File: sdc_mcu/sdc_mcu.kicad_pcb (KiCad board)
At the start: 2 copper layers, 70 x 45 mm, 93 parts, among them J1 Conn_02x10_Odd_Even, K1 G2RL-2A, K2 G2RL-2A, K3 G2RL-2A, K4 G2RL-2A, Q1 2N7002, Q2 2N7002, Q3 2N7002, Q4 2N7002, Q5 2N7002, Q6 2N7002, U1 VOM618AT, U10 AP2204K-ADJ, U2 VOM618AT, U3 AS331KTR-G1, U4 AS331KTR-G1, U5 AS331KTR-G1, U6 VOM618AT, U7 VOM618AT, U9 AP2204K-ADJ

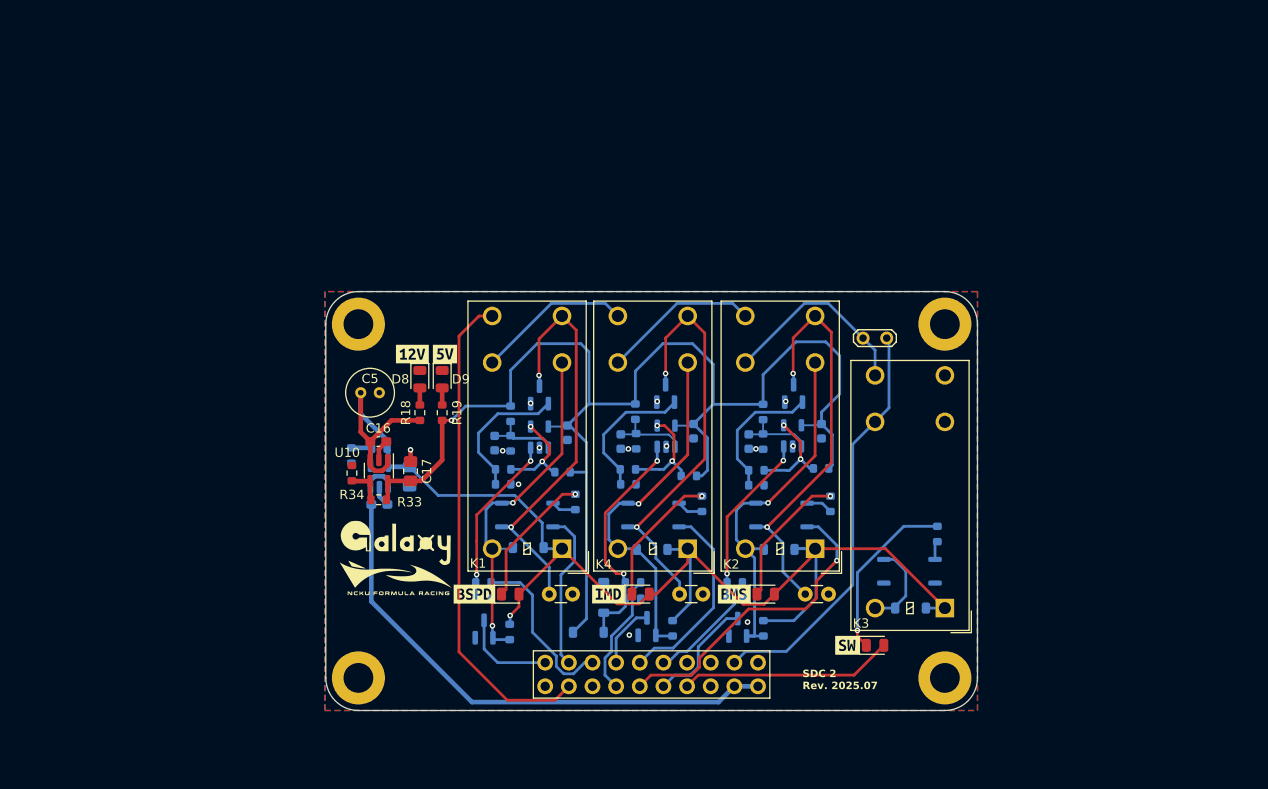
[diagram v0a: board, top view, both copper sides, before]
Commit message: v2025.10
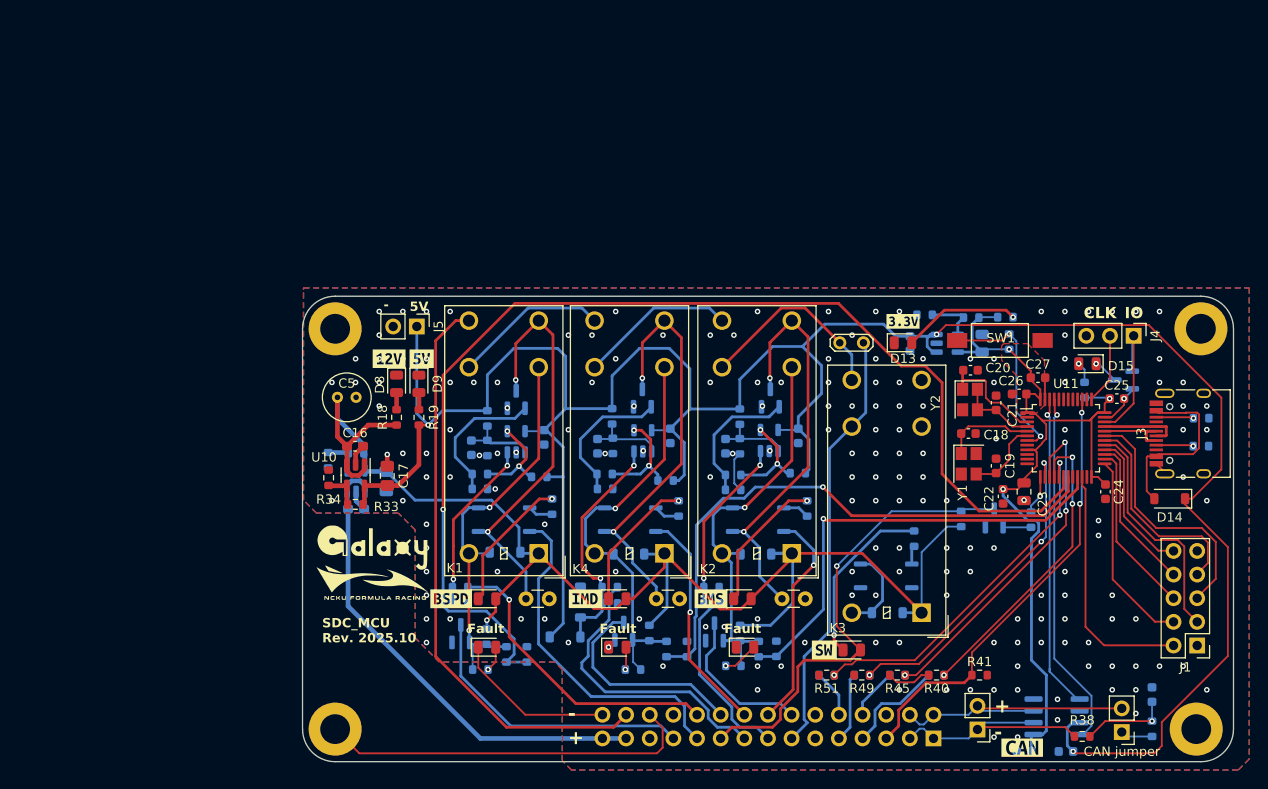
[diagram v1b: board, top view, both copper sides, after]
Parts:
- added C18: 20p, Capacitor_SMD:C_0603_1608Metric, F.Cu at (122.0, 63.2)
- added C19: 20p, Capacitor_SMD:C_0603_1608Metric, F.Cu at (125.0, 66.7)
- added C20: 20p, Capacitor_SMD:C_0603_1608Metric, F.Cu at (122.2, 56.5)
- added C21: 20p, Capacitor_SMD:C_0603_1608Metric, F.Cu at (125.0, 60.0)
- added C22: 100n, Capacitor_SMD:C_0603_1608Metric, F.Cu at (125.8, 70.0)
- added C23: 10u, Capacitor_SMD:C_0805_2012Metric, F.Cu at (128.0, 69.5)
- added C24: 100n, Capacitor_SMD:C_0603_1608Metric, F.Cu at (136.8, 69.5)
- added C25: 100n, Capacitor_SMD:C_0603_1608Metric, F.Cu at (138.0, 59.5)
- added C26: 100n, Capacitor_SMD:C_0603_1608Metric, F.Cu at (127.5, 59.0)
- added C27: 100n, Capacitor_SMD:C_0603_1608Metric, F.Cu at (129.5, 57.2)
- added C28: 1u, Capacitor_SMD:C_0603_1608Metric, B.Cu at (115.8, 53.6)
- added C29: 10u, Capacitor_SMD:C_0805_2012Metric, B.Cu at (123.5, 53.5)
- added C6: 100n, Capacitor_SMD:C_0603_1608Metric, B.Cu at (128.0, 97.4)
- added C7: 100n, Capacitor_SMD:C_0603_1608Metric, B.Cu at (132.5, 97.4)
- added C8: 1u, Capacitor_SMD:C_0603_1608Metric, B.Cu at (141.8, 91.3)
- added D13: PWR, LED_SMD:LED_0805_2012Metric, F.Cu at (115.0, 53.5)
- added D14: BAT46W-7-F, Diode_SMD:D_SOD-123, F.Cu at (143.7, 70.2)
- added D15: LED, LED_SMD:LED_0805_2012Metric, F.Cu at (134.8, 55.8)
- added D16: ~, LED_SMD:LED_0805_2012Metric, F.Cu at (70.3, 86.2)
- added D17: ~, LED_SMD:LED_0805_2012Metric, F.Cu at (98.0, 86.2)
- added D18: ~, LED_SMD:LED_0805_2012Metric, F.Cu at (84.3, 86.2)
- added J3: USB_C_Receptacle_USB2.0_16P, Connector_USB:USB_C_Receptacle_HRO_TYPE-C-31-M-12, F.Cu at (146.2, 63.2)
- added J4: Conn_01x03_Pin, Connector_PinHeader_2.54mm:PinHeader_1x03_P2.54mm_Vertical, F.Cu at (139.8, 52.8)
- added J5: Conn_01x02_Pin, Connector_PinHeader_2.54mm:PinHeader_1x02_P2.54mm_Vertical, F.Cu at (62.8, 51.8)
- added J6: Conn_01x02_Pin, Connector_PinHeader_2.54mm:PinHeader_1x02_P2.54mm_Vertical, F.Cu at (123.0, 95.0)
- added J7: Conn_02x15_Odd_Even, Connector_PinHeader_2.54mm:PinHeader_2x15_P2.54mm_Vertical, B.Cu at (118.3, 96.0)
- added JP2: Jumper_2_Open, Connector_PinHeader_2.54mm:PinHeader_1x02_P2.54mm_Vertical, F.Cu at (138.5, 95.3)
- added Q7: 2N7002, Package_TO_SOT_SMD:SOT-23, B.Cu at (124.8, 72.3)
- added Q8: 2N7002, Package_TO_SOT_SMD:SOT-23, B.Cu at (138.7, 57.5)
- added R35: 47k, Resistor_SMD:R_0603_1608Metric, B.Cu at (72.4, 87.0)
- added R36: 100k, Resistor_SMD:R_0603_1608Metric, B.Cu at (74.6, 87.0)
- added R37: 60R, Resistor_SMD:R_0603_1608Metric, B.Cu at (141.8, 95.0)
- added R38: 60R, Resistor_SMD:R_0603_1608Metric, F.Cu at (134.2, 95.8)
- added R39: 47k, Resistor_SMD:R_0603_1608Metric, B.Cu at (118.6, 89.2)
- added R40: 100k, Resistor_SMD:R_0603_1608Metric, F.Cu at (118.6, 89.2)
- added R41: 47k, Resistor_SMD:R_0603_1608Metric, F.Cu at (123.2, 89.2)
- added R42: 47k, Resistor_SMD:R_0603_1608Metric, B.Cu at (99.5, 86.4)
- added R43: 100k, Resistor_SMD:R_0603_1608Metric, B.Cu at (101.4, 86.4)
- added R44: 47k, Resistor_SMD:R_0603_1608Metric, B.Cu at (114.4, 89.2)
- added R45: 100k, Resistor_SMD:R_0603_1608Metric, F.Cu at (114.4, 89.2)
- added R46: 47k, Resistor_SMD:R_0603_1608Metric, B.Cu at (89.6, 86.4)
- added R47: 100k, Resistor_SMD:R_0603_1608Metric, B.Cu at (91.8, 86.4)
- added R48: 47k, Resistor_SMD:R_0603_1608Metric, B.Cu at (110.6, 89.2)
- added R49: 100k, Resistor_SMD:R_0603_1608Metric, F.Cu at (110.6, 89.2)
- added R50: 47k, Resistor_SMD:R_0603_1608Metric, B.Cu at (106.8, 89.2)
- added R51: 100k, Resistor_SMD:R_0603_1608Metric, F.Cu at (106.8, 89.2)
- added R52: 5k1, Resistor_SMD:R_0603_1608Metric, B.Cu at (147.0, 61.6)
- added R53: 5k1, Resistor_SMD:R_0603_1608Metric, B.Cu at (147.0, 64.6)
- added R54: 100k, Resistor_SMD:R_0603_1608Metric, B.Cu at (117.3, 50.5)
- added R55: 165k, Resistor_SMD:R_0603_1608Metric, B.Cu at (122.3, 50.8)
- added R56: 4.7k, Resistor_SMD:R_0603_1608Metric, B.Cu at (128.8, 72.5)
- added R57: 10k, Resistor_SMD:R_0603_1608Metric, B.Cu at (121.2, 72.4)
- added R58: 10k, Resistor_SMD:R_0603_1608Metric, B.Cu at (126.4, 53.4)
- added R59: 10k, Resistor_SMD:R_0603_1608Metric, B.Cu at (126.0, 50.8)
- added R60: 10k, Resistor_SMD:R_0603_1608Metric, B.Cu at (134.5, 58.6)
- added R61: 10k, Resistor_SMD:R_0603_1608Metric, B.Cu at (69.6, 88.6)
- added R62: 10k, Resistor_SMD:R_0603_1608Metric, B.Cu at (96.8, 88.2)
- added R63: 10k, Resistor_SMD:R_0603_1608Metric, B.Cu at (86.0, 88.6)
- added SW1: SW_SPST, Button_Switch_SMD:SW_SPST_FSMSM, F.Cu at (125.4, 53.2)
- added U11: STM32F103C8Tx, Package_QFP:LQFP-48_7x7mm_P0.5mm, F.Cu at (132.5, 63.8)
- added U12: AP2204K-ADJ, Package_TO_SOT_SMD:SOT-23-5, B.Cu at (119.8, 53.5)
- added U8: SN65HVD256D, Package_SO:SOIC-8_3.9x4.9mm_P1.27mm, B.Cu at (131.5, 93.7)
- added Y1: 8M, Crystal:Crystal_SMD_SeikoEpson_FA238-4Pin_3.2x2.5mm, F.Cu at (122.1, 66.5)
- added Y2: 32.768k, Crystal:Crystal_SMD_SeikoEpson_FA238-4Pin_3.2x2.5mm, F.Cu at (122.2, 59.6)
- added kibuzzard-68E9BB8F: G***, kibuzzard-68E9BB8F, F.Cu at (127.8, 97.0)
- added kibuzzard-68E9BC03: G***, kibuzzard-68E9BC03, F.Cu at (115.0, 51.2)
- J1: value Conn_02x10_Odd_Even -> Conn_02x05_Odd_Even; footprint Connector_PinHeader_2.54mm:PinHeader_2x10_P2.54mm_Vertical -> Connector_PinHeader_2.54mm:PinHeader_2x05_P2.54mm_Vertical
- R18, R19: value 1k -> 10k
- moved J1 47.2 mm to (146.6, 86.0), turned to 180 degrees
- moved H2 27.6 mm to (146.5, 95.0)
- moved H3 27.5 mm to (147.0, 52.0)
- moved H4 6.04 mm to (54.0, 95.0)
- moved C1 2.55 mm to (68.6, 64.8)
- moved C10 2.55 mm to (76.5, 63.7)
- moved C11 2.55 mm to (88.5, 81.0)
- moved C12 2.55 mm to (74.5, 81.0)
- moved C13 2.55 mm to (102.0, 81.0)
- moved C14 2.55 mm to (56.2, 71.4)
- moved C15 2.55 mm to (59.5, 68.4)
- moved C16 2.55 mm to (56.1, 64.6)
- moved C17 2.55 mm to (59.6, 67.8)
- moved C2 2.55 mm to (95.9, 64.6)
- moved C3 2.55 mm to (90.0, 63.5)
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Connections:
- J1 pad 10: BMS_LED -> PB15
- J1 pad 2: VDC -> PB11
- J1 pad 3: SW_OUT -> PA8
- J1 pad 4: VDC -> PB12
- J1 pad 5: GND -> PA10
- J1 pad 6: unconnected-(J1-Pin_6-Pad6) -> PB13
- J1 pad 7: GND -> PA9
- J1 pad 8: SW_Fault -> PB14
- J1 pad 9: BMS_FAULT -> GND
- JP1 pad 2: SW_OUT -> SDC_OUT
- K3 pad 23: SW_OUT -> SDC_OUT
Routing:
- net BSPD_LED_MCU: track 0.00 -> 126.0 mm, vias 0 -> 1
- net +5V: track 141.4 -> 265.2 mm, vias 1 -> 3
- net +3.3V: track 0.00 -> 89.1 mm, vias 0 -> 3
- net GND: track 5.79 -> 82.0 mm, vias 13 -> 177
- net IMD_LED_MCU: track 0.00 -> 62.3 mm, vias 0 -> 1
- net BMS_LED_MCU: track 0.00 -> 48.8 mm, vias 0 -> 1
- net TSSI: track 0.00 -> 47.5 mm, vias 0 -> 2
- net SDC_OUT: track 0.00 -> 46.2 mm
- net SW_OUT: track 44.4 -> 0.00 mm
- net CAN_RX: track 0.00 -> 38.6 mm, vias 0 -> 1
- net BSPD_Check4: track 0.00 -> 38.5 mm, vias 0 -> 3
- net BSPD_Check2: track 0.00 -> 37.3 mm, vias 0 -> 3
- net BSPD_Check3: track 0.00 -> 34.7 mm, vias 0 -> 3
- net CAN_TX: track 0.00 -> 33.9 mm, vias 0 -> 1
- net BSPD_Check1: track 0.00 -> 33.0 mm, vias 0 -> 3
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- added copper zone on F.Cu, net +3.3V
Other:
- board size 70 x 45 mm -> 100 x 50 mm
- board text added: "+"
- board text added: "-"
- board text added: "5V"
- board text added: "CAN jumper"
- board text added: "CLK"
- board text added: "Fault"
- board text added: "IO"
- board text added: "SDC_MCU Rev. 2025.10"
- board text removed: "SDC 2 Rev. 2025.07"

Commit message: feat: relayout sdc mcu
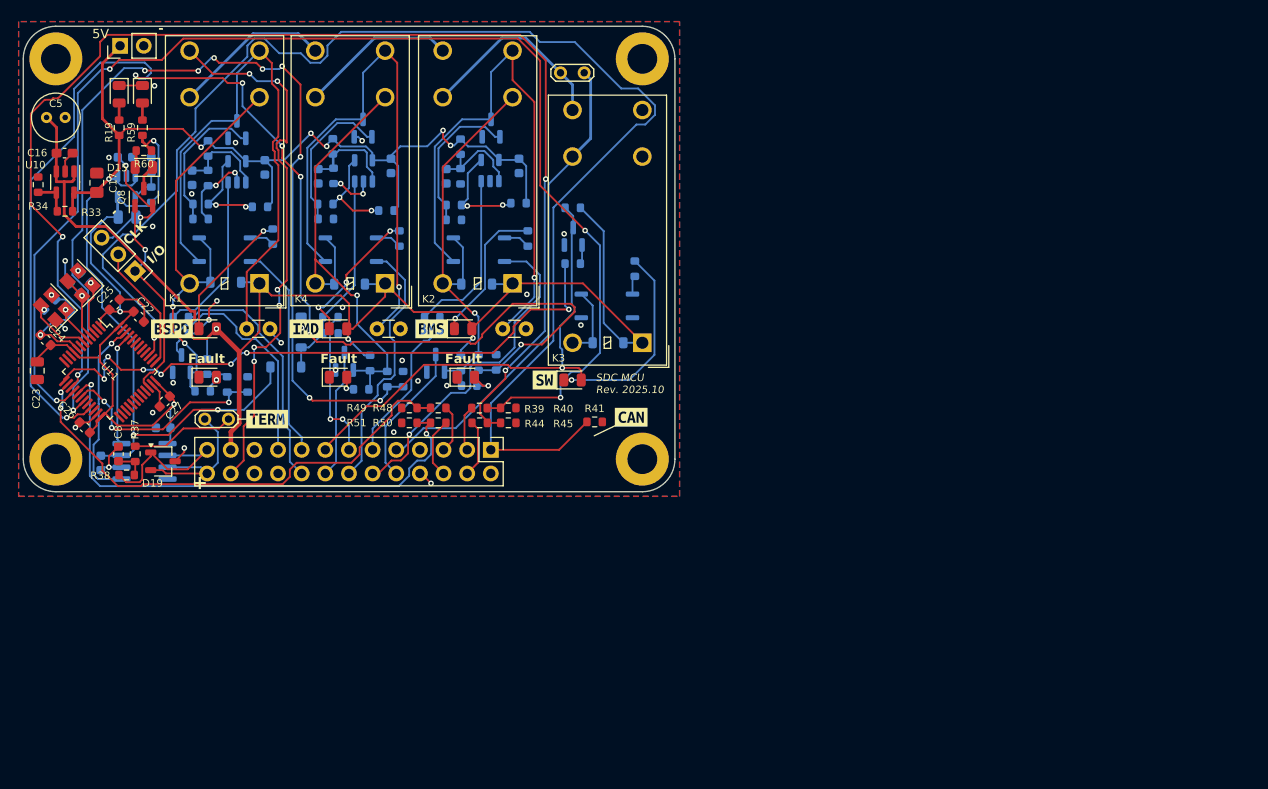
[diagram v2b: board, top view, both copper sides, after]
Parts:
- removed C14: 1u, Capacitor_SMD:C_0603_1608Metric_Pad1.08x0.95mm_HandSolder
- removed C15: 10u, Capacitor_SMD:C_0805_2012Metric_Pad1.18x1.45mm_HandSolder
- removed D14: BAT46W-7-F, Diode_SMD:D_SOD-123
- removed D8: PWR, LED_SMD:LED_0805_2012Metric
- removed J1: Conn_02x05_Odd_Even, Connector_PinHeader_2.54mm:PinHeader_2x05_P2.54mm_Vertical
- removed J3: USB_C_Receptacle_USB2.0_16P, Connector_USB:USB_C_Receptacle_HRO_TYPE-C-31-M-12
- removed J6: Conn_01x02_Pin, Connector_PinHeader_2.54mm:PinHeader_1x02_P2.54mm_Vertical
- removed J7: Conn_02x15_Odd_Even, Connector_PinHeader_2.54mm:PinHeader_2x15_P2.54mm_Vertical
- removed R18, R58: 10k, Resistor_SMD:R_0603_1608Metric
- removed R31: 866k, Resistor_SMD:R_0603_1608Metric
- removed R32: 100k, Resistor_SMD:R_0603_1608Metric
- removed R52, R53: 5k1, Resistor_SMD:R_0603_1608Metric
- removed SW1: SW_SPST, Button_Switch_SMD:SW_SPST_FSMSM
- removed U9: AP2204K-ADJ, Package_TO_SOT_SMD:SOT-23-5
- removed kibuzzard-67515DEB: G***, kibuzzard-67515DEB
- removed kibuzzard-67515DF6: G***, kibuzzard-67515DF6
- removed kibuzzard-68E9BB8F: G***, kibuzzard-68E9BB8F
- removed kibuzzard-68E9BC03: G***, kibuzzard-68E9BC03
- added D19: DESD2CAN2SOQ, Package_TO_SOT_SMD:TSOT-23, F.Cu at (35.5, 66.2)
- added J2: Conn_02x13_Odd_Even, Connector_PinHeader_2.54mm:PinHeader_2x13_P2.54mm_Vertical, F.Cu at (70.7, 65.0)
- added kibuzzard-68EF6159: G***, kibuzzard-68EF6159, F.Cu at (46.7, 61.7)
- added kibuzzard-68EF6180: G***, kibuzzard-68EF6180, F.Cu at (85.8, 61.5)
- C18, C19, C20, C21: moved to B.Cu
- C8, Q8, R37, R39, R44, R48, R50, R59, R60: moved to F.Cu
- G1, G2: renamed from G***; moved to B.Cu
- JP2: footprint Connector_PinHeader_2.54mm:PinHeader_1x02_P2.54mm_Vertical -> TestPoint:TestPoint_2Pads_Pitch2.54mm_Drill0.8mm
- moved C24 115.0 mm to (22.9, 53.2), turned to 135 degrees
- moved C8 114.0 mm to (30.7, 65.4)
- moved R37 113.1 mm to (32.5, 65.4), turned to -90 degrees
- moved C7 108.2 mm to (28.8, 66.4), turned to -90 degrees
- moved C25 108.1 mm to (30.3, 49.4), turned to 45 degrees
- moved J4 107.5 mm to (32.5, 45.8), turned to -135 degrees
- moved Q8 107.1 mm to (33.5, 37.9), turned to 90 degrees
- moved C23 106.8 mm to (22.0, 56.5)
- moved R38 106.4 mm to (31.6, 67.7)
- moved R60 104.3 mm to (33.5, 32.9), turned to 180 degrees
- moved JP2 104.1 mm to (40.0, 61.7), turned to 0 degrees
- moved D15 103.5 mm to (33.5, 34.7)
- moved C19 103.0 mm to (23.3, 50.5), turned to -45 degrees
- moved U11 102.9 mm to (29.8, 56.6), turned to -45 degrees
- moved U8 101.7 mm to (33.5, 66.2), turned to 0 degrees
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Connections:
- net +3.3V renamed +3V3
- JP2 pad 1: Net-(JP2-A) -> CAN+
- JP2 pad 2: CAN+ -> Net-(JP2-B)
- R37 pad 1: Net-(JP2-A) -> Net-(JP2-B)
- U11 pad 7: Net-(SW1-B) -> unconnected-(U11-NRST-Pad7)
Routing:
- net +5V: track 265.2 -> 155.7 mm, vias 3 -> 8
- net BSPD_Check1: track 33.0 -> 141.1 mm, vias 3 -> 4
- net TSSI: track 47.5 -> 149.8 mm, vias 2 -> 1
- net BSPD_LED_MCU: track 126.0 -> 23.8 mm, vias 1 -> 3
- net BSPD_Check2: track 37.3 -> 137.2 mm, vias 3 -> 4
- net BMS_LED_MCU: track 48.8 -> 140.9 mm, vias 1 -> 7
- net SW_Signal: track 4.18 -> 66.6 mm, vias 1 -> 7
- net VDC: track 51.7 -> 0.00 mm
- net IMD_LED_MCU: track 62.3 -> 109.1 mm, vias 1 -> 9
- net PA10: track 27.2 -> 0.00 mm
- net PB11: track 26.5 -> 0.00 mm
- net CAN_RX: track 38.6 -> 12.3 mm
- net PA8: track 25.2 -> 0.00 mm
- net PA9: track 23.0 -> 0.00 mm
- net PB12: track 21.1 -> 0.00 mm
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- removed copper zone on F.Cu, net +3V3
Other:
- board size 100 x 50 mm -> 70 x 50 mm
- board text added: "- CLK I/O"
- board text added: "SDC MCU Rev. 2025.10"
- board text removed: "CAN jumper"
- board text removed: "CLK"
- board text removed: "IO"
- board text removed: "SDC_MCU Rev. 2025.10"
